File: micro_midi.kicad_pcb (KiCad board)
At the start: 2 copper layers, 67 parts, among them U1 74HC595, U2 Arduino_Micro, U3 74HC595

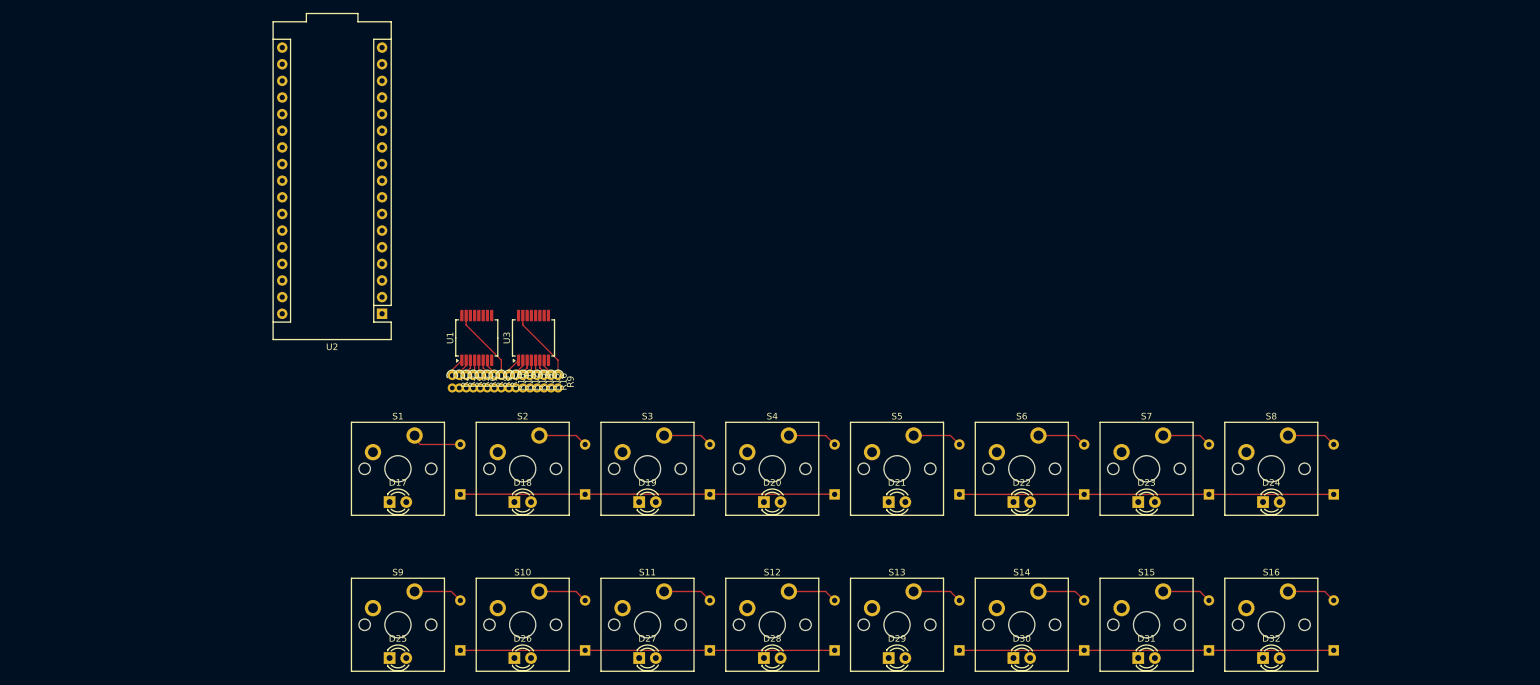
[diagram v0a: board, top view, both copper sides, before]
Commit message: nearing completion
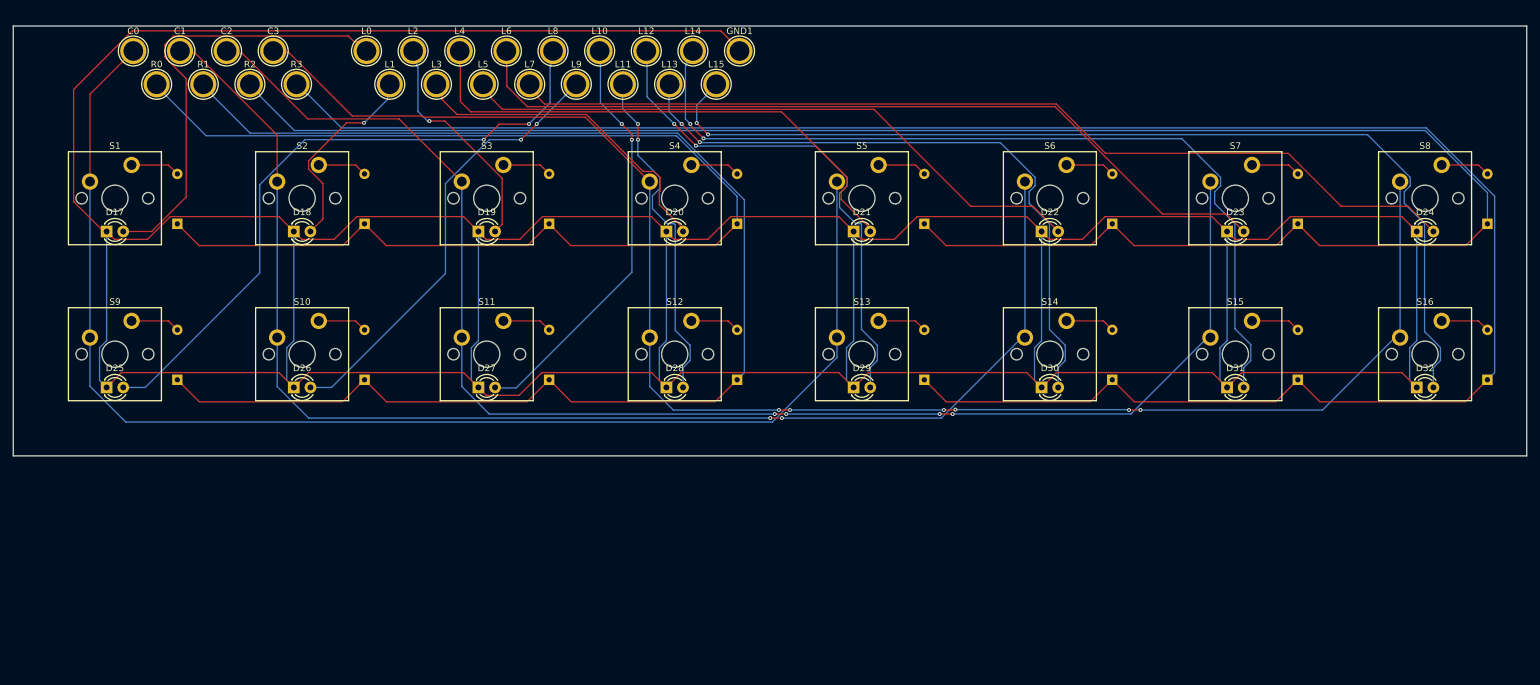
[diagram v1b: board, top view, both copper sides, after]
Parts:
- removed R10, R11, R12, R13, R14, R15, R16, R4, R5, R6, R7, R8, R9: Resistor, Resistor_THT:R_Axial_DIN0204_L3.6mm_D1.6mm_P1.90mm_Vertical
- removed U1, U3: 74HC595, Package_SO:SSOP-16_5.3x6.2mm_P0.65mm
- removed U2: Arduino_Micro, Arduino:Arduino_Micro
- added C0: MountingHole_Pad, TestPoint:TestPoint_Plated_Hole_D3.0mm, F.Cu at (49.8, 49.8)
- added C1: MountingHole_Pad, TestPoint:TestPoint_Plated_Hole_D3.0mm, F.Cu at (57.0, 49.8)
- added C2: MountingHole_Pad, TestPoint:TestPoint_Plated_Hole_D3.0mm, F.Cu at (64.1, 49.8)
- added C3: MountingHole_Pad, TestPoint:TestPoint_Plated_Hole_D3.0mm, F.Cu at (71.2, 49.8)
- added GND1: MountingHole_Pad, TestPoint:TestPoint_Plated_Hole_D3.0mm, F.Cu at (142.4, 49.8)
- added L0: MountingHole_Pad, TestPoint:TestPoint_Plated_Hole_D3.0mm, F.Cu at (85.4, 49.8)
- added L1: MountingHole_Pad, TestPoint:TestPoint_Plated_Hole_D3.0mm, F.Cu at (89.0, 54.9)
- added L10: MountingHole_Pad, TestPoint:TestPoint_Plated_Hole_D3.0mm, F.Cu at (121.0, 49.8)
- added L11: MountingHole_Pad, TestPoint:TestPoint_Plated_Hole_D3.0mm, F.Cu at (124.6, 54.9)
- added L12: MountingHole_Pad, TestPoint:TestPoint_Plated_Hole_D3.0mm, F.Cu at (128.2, 49.8)
- added L13: MountingHole_Pad, TestPoint:TestPoint_Plated_Hole_D3.0mm, F.Cu at (131.7, 54.9)
- added L14: MountingHole_Pad, TestPoint:TestPoint_Plated_Hole_D3.0mm, F.Cu at (135.3, 49.8)
- added L15: MountingHole_Pad, TestPoint:TestPoint_Plated_Hole_D3.0mm, F.Cu at (138.8, 54.9)
- added L2: MountingHole_Pad, TestPoint:TestPoint_Plated_Hole_D3.0mm, F.Cu at (92.6, 49.8)
- added L3: MountingHole_Pad, TestPoint:TestPoint_Plated_Hole_D3.0mm, F.Cu at (96.1, 54.9)
- added L4: MountingHole_Pad, TestPoint:TestPoint_Plated_Hole_D3.0mm, F.Cu at (99.7, 49.8)
- added L5: MountingHole_Pad, TestPoint:TestPoint_Plated_Hole_D3.0mm, F.Cu at (103.2, 54.9)
- added L6: MountingHole_Pad, TestPoint:TestPoint_Plated_Hole_D3.0mm, F.Cu at (106.8, 49.8)
- added L7: MountingHole_Pad, TestPoint:TestPoint_Plated_Hole_D3.0mm, F.Cu at (110.4, 54.9)
- added L8: MountingHole_Pad, TestPoint:TestPoint_Plated_Hole_D3.0mm, F.Cu at (113.9, 49.8)
- added L9: MountingHole_Pad, TestPoint:TestPoint_Plated_Hole_D3.0mm, F.Cu at (117.5, 54.9)
- added R0: MountingHole_Pad, TestPoint:TestPoint_Plated_Hole_D3.0mm, F.Cu at (53.4, 54.9)
- R1, R2, R3: value Resistor -> MountingHole_Pad; footprint Resistor_THT:R_Axial_DIN0204_L3.6mm_D1.6mm_P1.90mm_Vertical -> TestPoint:TestPoint_Plated_Hole_D3.0mm
- moved R1 63.6 mm to (60.5, 54.9), turned to 0 degrees
- moved D25 59.8 mm to (45.8, 101.2)
- moved S1 59.8 mm to (47.0, 72.3)
- moved S9 59.8 mm to (47.0, 96.1)
- moved D1 59.8 mm to (56.6, 76.2)
- moved D17 59.8 mm to (45.8, 77.4)
- moved D9 59.8 mm to (56.6, 100.0)
- moved R2 54.1 mm to (67.6, 54.9), turned to 0 degrees
- moved D26 53.3 mm to (74.3, 101.2)
- moved D18 53.3 mm to (74.3, 77.4)
- moved S10 53.3 mm to (75.6, 96.1)
- moved S2 53.3 mm to (75.6, 72.3)
- moved D10 53.3 mm to (85.1, 100.0)
- moved D2 53.3 mm to (85.1, 76.2)
- moved R3 50.9 mm to (74.8, 54.9), turned to 0 degrees
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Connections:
- net /COL 0 renamed Net-(C0-Pad1)
- net /COL 1 renamed Net-(C1-Pad1)
- net /COL 2 renamed Net-(C2-Pad1)
- net /COL 3 renamed Net-(C3-Pad1)
- net /ROW 0 renamed Net-(D1-K)
- net GND renamed Net-(D17-K)
- D10 pad 1: /ROW 1 -> Net-(D10-K)
- D11 pad 1: /ROW 1 -> Net-(D10-K)
- D12 pad 1: /ROW 1 -> Net-(D10-K)
- D13 pad 1: /ROW 3 -> Net-(D13-K)
- D14 pad 1: /ROW 3 -> Net-(D13-K)
- D15 pad 1: /ROW 3 -> Net-(D13-K)
- D16 pad 1: /ROW 3 -> Net-(D13-K)
- D5 pad 1: /ROW 2 -> Net-(D5-K)
- D6 pad 1: /ROW 2 -> Net-(D5-K)
- D7 pad 1: /ROW 2 -> Net-(D5-K)
- D8 pad 1: /ROW 2 -> Net-(D5-K)
- D9 pad 1: /ROW 1 -> Net-(D10-K)
- R1 pad 1: Net-(U1-QA) -> Net-(D10-K)
- R2 pad 1: Net-(U1-QB) -> Net-(D5-K)
- R3 pad 1: Net-(U1-QC) -> Net-(D13-K)
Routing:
- net Net-(D17-K): track 0.00 -> 762.9 mm
- net Net-(D13-K): track 0.00 -> 312.8 mm
- net Net-(D5-K): track 0.00 -> 295.1 mm
- net Net-(C3-Pad1): track 0.00 -> 241.5 mm, vias 0 -> 6
- net Net-(C2-Pad1): track 0.00 -> 220.2 mm, vias 0 -> 4
- net Net-(D10-K): track 0.00 -> 211.9 mm
- net Net-(C1-Pad1): track 0.00 -> 203.6 mm, vias 0 -> 2
- net Net-(C0-Pad1): track 0.00 -> 201.2 mm
- net Net-(D32-A): track 0.00 -> 154.7 mm, vias 0 -> 2
- net Net-(D24-A): track 0.00 -> 147.7 mm
- net Net-(D1-K): track 57.2 -> 193.8 mm
- net Net-(D31-A): track 0.00 -> 131.6 mm, vias 0 -> 2
- net Net-(D23-A): track 0.00 -> 127.1 mm
- net Net-(D30-A): track 0.00 -> 99.4 mm, vias 0 -> 2
- net Net-(D25-A): track 0.00 -> 99.2 mm, vias 0 -> 2
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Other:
- board outline added: 231.1 x 65.6 mm
